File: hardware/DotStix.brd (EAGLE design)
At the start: 20.3 x 50 mm, 20 parts, among them U1 ATMEGA328P-MU-QFN32

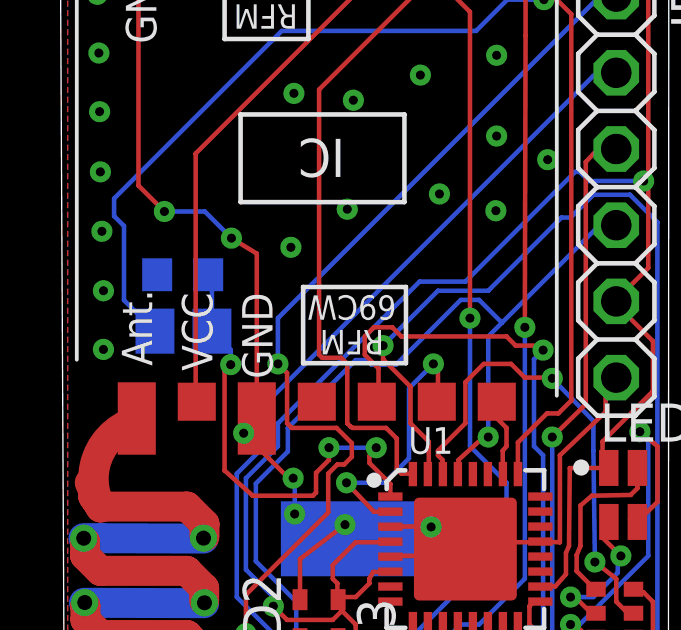
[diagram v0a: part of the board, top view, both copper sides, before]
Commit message: Minor info improvements
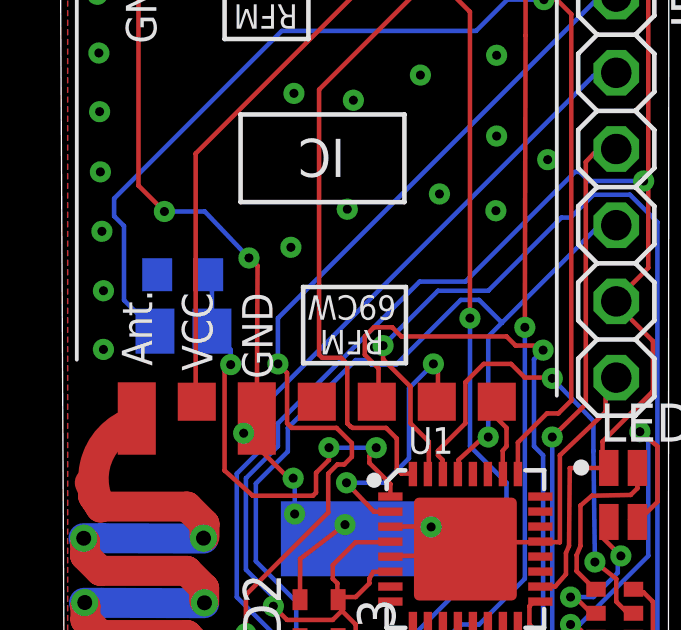
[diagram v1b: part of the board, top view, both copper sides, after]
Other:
- board text added: "If you plan on potting the board in transparent epoxy, the battery's max cycle count ist 1000. Use a 330mF Supercap instead of battery: DSK-3R3H334T-HL"
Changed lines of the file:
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@@
 <setting verticaltext="up"/>
 </settings>
-<grid distance="1" unitdist="mil" unit="mm" style="lines" multiple="1" display="yes" altdistance="0.025" altunitdist="inch" altunit="inch"/>
+<grid distance="0.00254" unitdist="mm" unit="mm" style="lines" multiple="1" display="yes" altdistance="0.025" altunitdist="inch" altunit="inch"/>
 <layers>
 <layer number="1" name="Top" color="4" fill="1" visible="yes" active="yes"/>
@@
 <layer number="45" name="Holes" color="7" fill="1" visible="no" active="yes"/>
 <layer number="46" name="Milling" color="3" fill="1" visible="no" active="yes"/>
-<layer number="47" name="Measures" color="7" fill="1" visible="no" active="yes"/>
+<layer number="47" name="Measures" color="7" fill="1" visible="yes" active="yes"/>
 <layer number="48" name="Document" color="7" fill="1" visible="yes" active="yes"/>
 <layer number="49" name="Reference" color="7" fill="1" visible="no" active="yes"/>
@@
 <text x="2.4892" y="17.145" size="1.016" layer="21" rot="SR90" align="center">HexID</text>
 <rectangle x1="1.3208" y1="20.066" x2="3.7592" y2="24.4856" layer="21"/>
+<text x="-0.06858125" y="59.93891875" size="1.778" layer="48">If you plan on potting the board in transparent epoxy, the battery's max cycle count ist 1000.
+Use a 330mF Supercap instead of battery: DSK-3R3H334T-HL  </text>
 </plain>
 <attributes>
@@
 <wire x1="12.1158" y1="28.0924" x2="10.1092" y2="28.0924" width="0.1524" layer="16"/>
 <wire x1="10.1092" y1="28.0924" x2="10.1092" y2="27.6968" width="0.1524" layer="16"/>
-<wire x1="6.3058" y1="31.7074" x2="6.3058" y2="37.2044" width="0.1524" layer="1"/>
-<wire x1="6.3058" y1="37.2044" x2="5.461" y2="37.719" width="0.1524" layer="1"/>
-<via x="5.461" y="37.719" extent="1-16" drill="0.3"/>
+<wire x1="6.3058" y1="31.7074" x2="6.3312" y2="36.798" width="0.1524" layer="1"/>
+<wire x1="6.3312" y1="36.798" x2="6.0452" y2="37.0586" width="0.1524" layer="1"/>
+<via x="6.0452" y="37.0586" extent="1-16" drill="0.3"/>
 <wire x1="2.3622" y1="48.2106" x2="2.3058" y2="48.267" width="0.1524" layer="1"/>
 <via x="17.4498" y="11.2776" extent="1-16" drill="0.3"/>
@@
 <via x="3.2258" y="38.608" extent="1-16" drill="0.3"/>
 <wire x1="3.2258" y1="38.608" x2="4.572" y2="38.608" width="0.1524" layer="16"/>
-<wire x1="4.572" y1="38.608" x2="5.461" y2="37.719" width="0.1524" layer="16"/>
+<wire x1="4.572" y1="38.608" x2="6.0452" y2="37.0586" width="0.1524" layer="16"/>
 <wire x1="7.5692" y1="28.5242" x2="7.5692" y2="29.6672" width="0.1524" layer="16"/>
 <wire x1="7.5692" y1="29.6672" x2="7.5184" y2="29.718" width="0.1524" layer="16"/>
